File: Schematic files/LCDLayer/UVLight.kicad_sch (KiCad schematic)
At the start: 50 parts, among them J1 Conn_01x03_Pin, Q1 NMOS

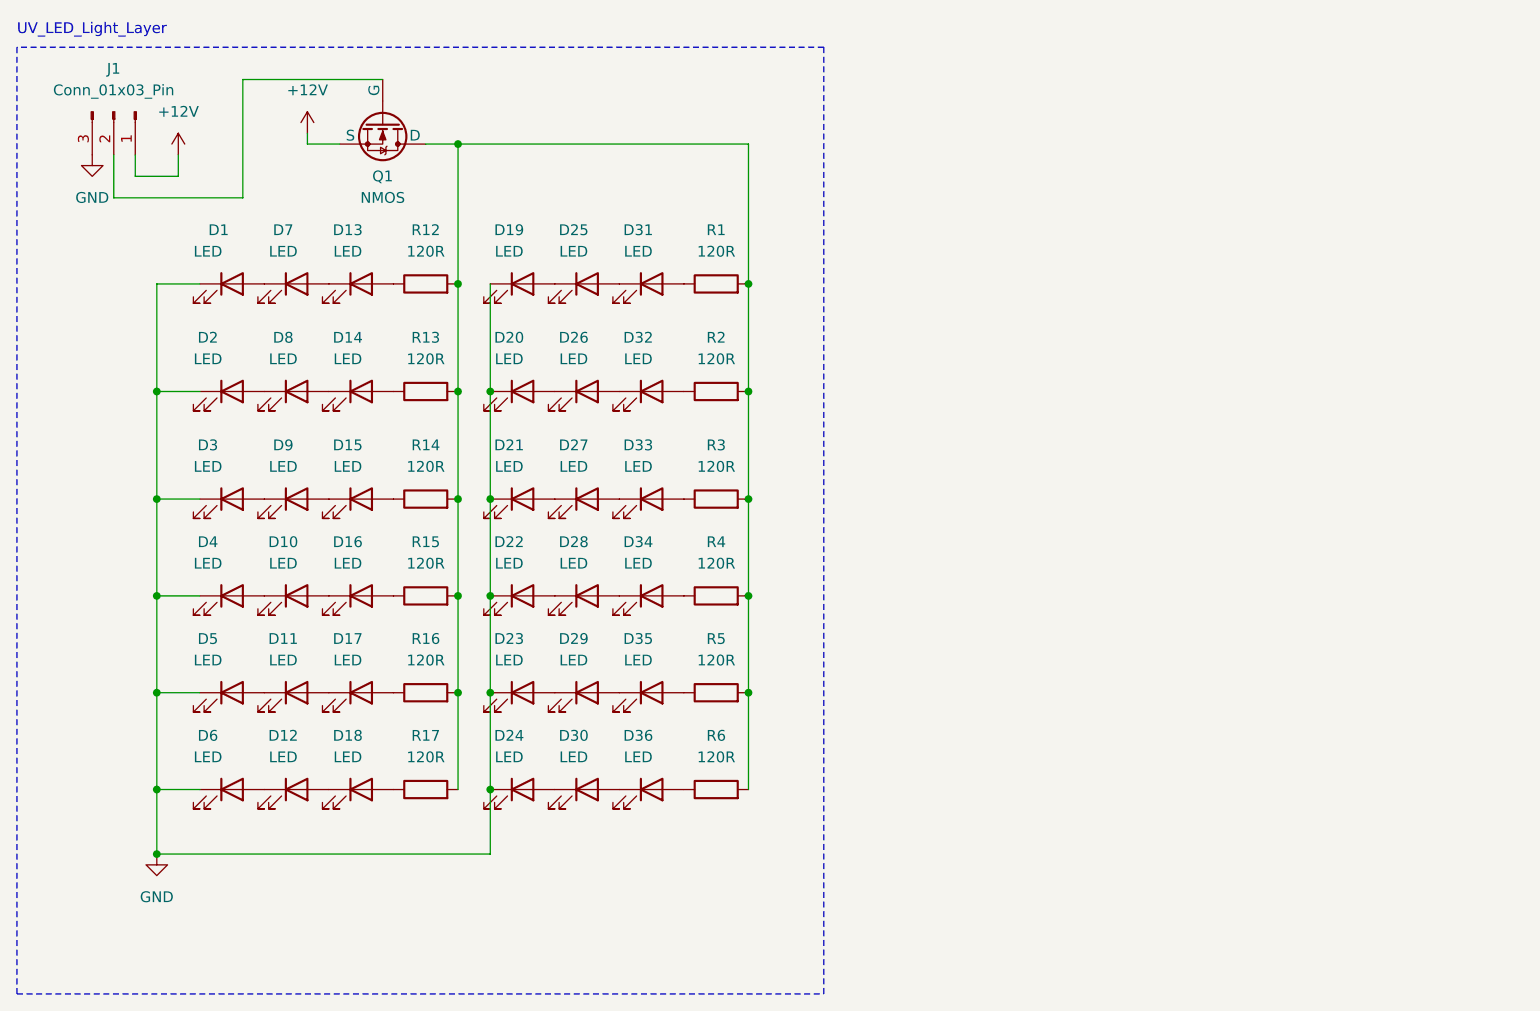
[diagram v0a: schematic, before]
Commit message: Finished Schematic
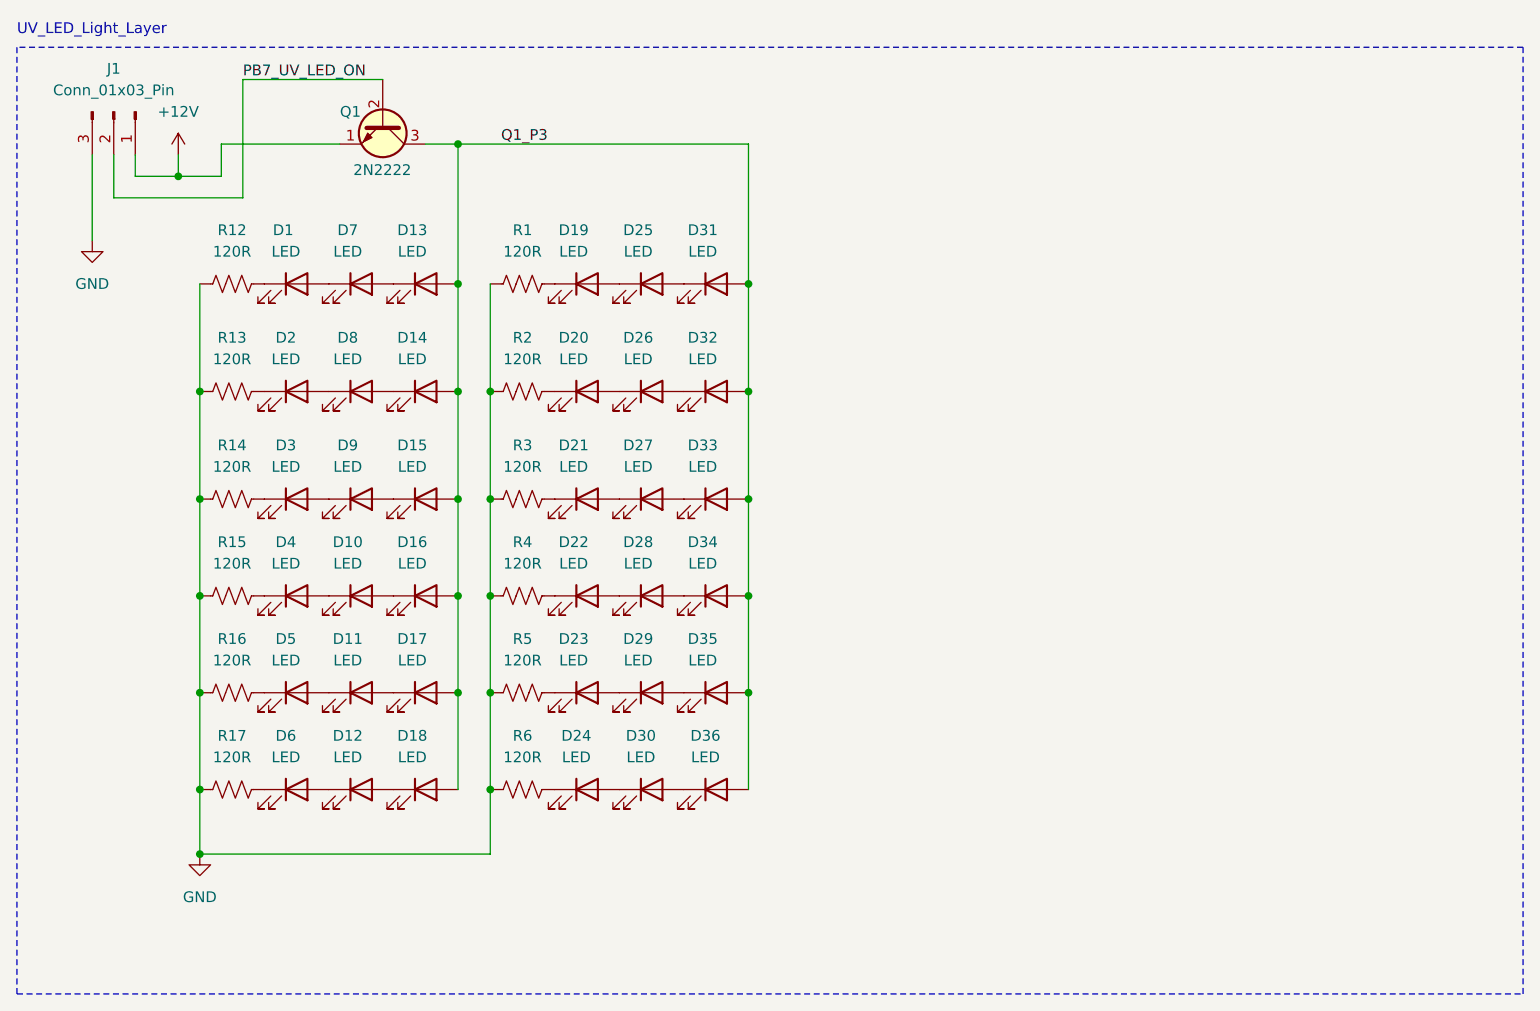
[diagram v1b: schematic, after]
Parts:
- removed Q1: NMOS, symbol Simulation_SPICE:NMOS
- added Q1: 2N2222, Package_TO_SOT_THT_AKL:TO-18-3_EBC, symbol PCM_Transistor_BJT_AKL:2N2222
- R1, R12, R13, R14, R15, R16, R17, R2, R3, R4, R5, R6: symbol Device:R -> Device:R_US
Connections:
- net +12V: now also Q1.1 (E)
- net GND: now also R1.1, R12.1, R13.1, R14.1, R15.1, R16.1, R17.1, R2.1, R3.1, R4.1, R5.1, R6.1; no longer D1.1 (K), D19.1 (K), D2.1 (K), D20.1 (K), D21.1 (K), D22.1 (K), D23.1 (K), D24.1 (K), D3.1 (K), D4.1 (K), D5.1 (K), D6.1 (K)
- net PB7_UV_LED_ON: now reaches J1.2 (Pin_2)
- net PB7_UV_LED_ON: now also Q1.2 (B)
- net Q1_P3: now reaches D31.2 (A)
- net Q1_P3: now also D13.2 (A), D14.2 (A), D15.2 (A), D16.2 (A), D17.2 (A), D18.2 (A), D32.2 (A), D33.2 (A), D34.2 (A), D35.2 (A), D36.2 (A), Q1.3 (C); no longer R1.1
- new net: D5.1 (K), R16.2
- new net: D4.1 (K), R15.2
- new net: D23.1 (K), R5.2
- new net: D1.1 (K), R12.2
- new net: D3.1 (K), R14.2
- new net: D6.1 (K), R17.2
- new net: D22.1 (K), R4.2
- new net: D19.1 (K), R1.2
- new net: D21.1 (K), R3.2
- new net: D24.1 (K), R6.2
- new net: D20.1 (K), R2.2
- new net: D2.1 (K), R13.2
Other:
- company: (none) -> Sidharth Sreeram
- title: (none) -> UVLED_Panel
- moved on the sheet: D1, D10, D11, D12, D13, D14, D15, D16, D17, D18, D19, D2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
